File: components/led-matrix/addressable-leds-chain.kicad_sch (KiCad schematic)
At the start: 90 parts

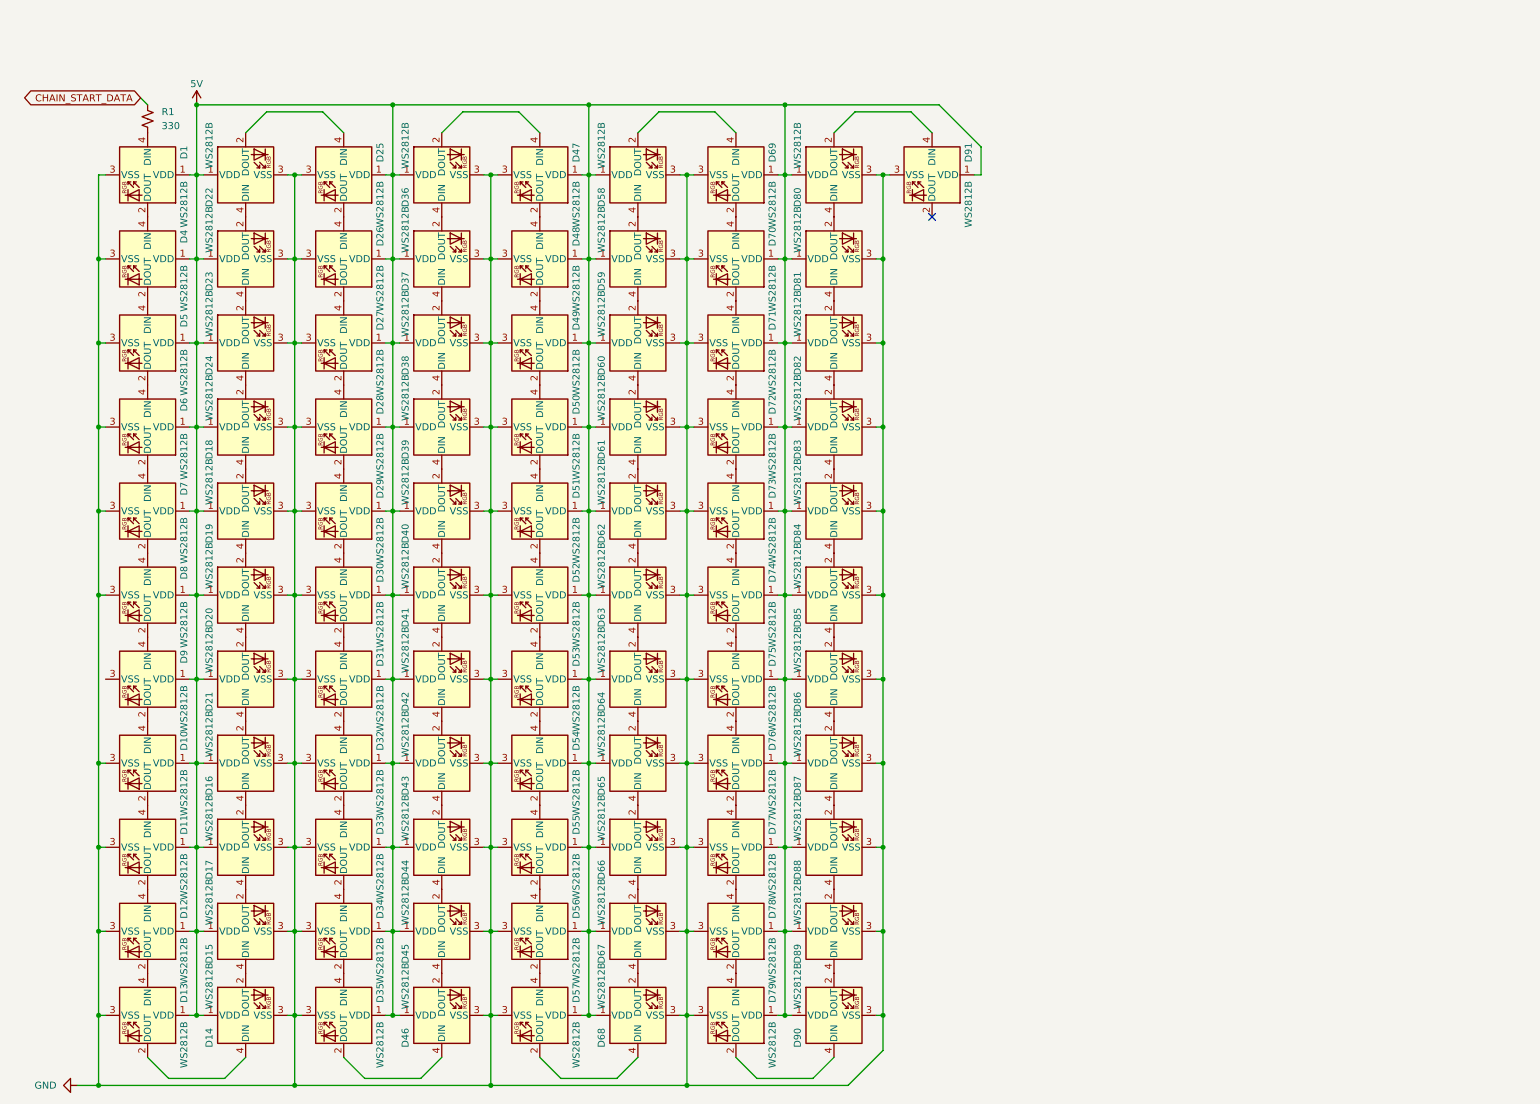
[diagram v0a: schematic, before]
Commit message: svg
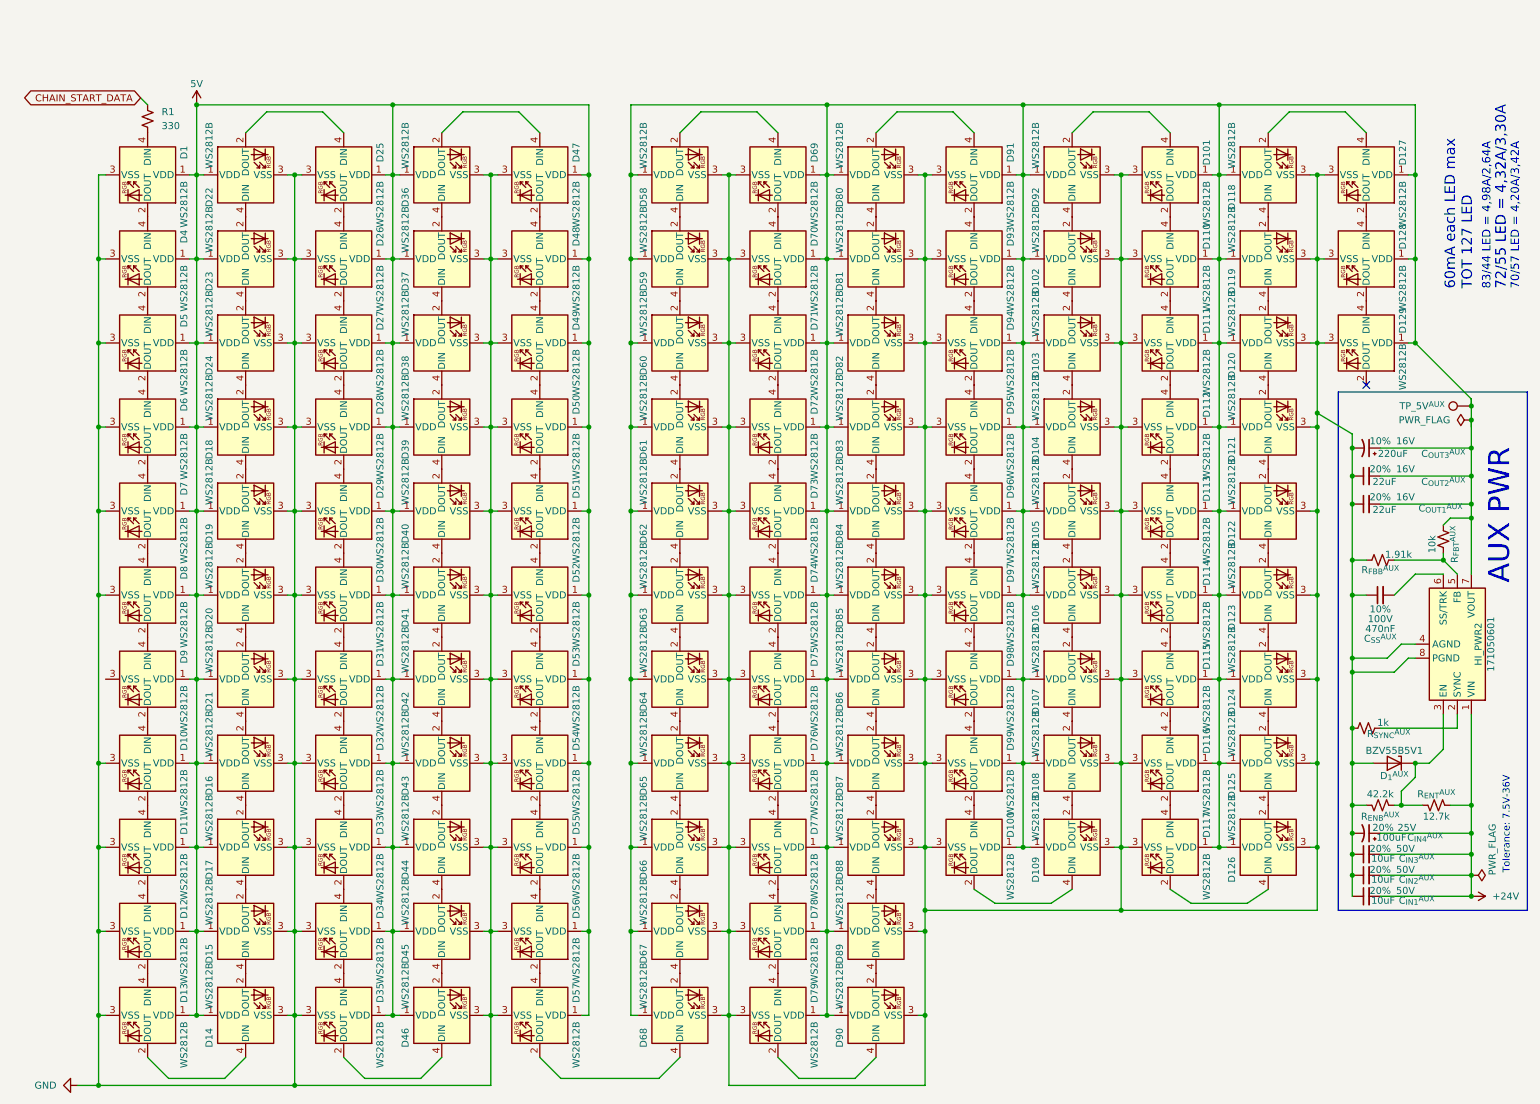
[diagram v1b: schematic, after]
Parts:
- added C_{IN1}^{AUX}, C_{IN2}^{AUX}, C_{IN3}^{AUX}: 10uF, PCM_SparkFun-Capacitor:C_1210_3225Metric, symbol PCM_SparkFun-Capacitor:10uF_1210_50V_20%
- added C_{IN4}^{AUX}: 100uF, PCM_SparkFun-Capacitor:Panasonic_D, symbol PCM_SparkFun-Capacitor:100uF_6.6x6.6_25V_20%
- added C_{OUT1}^{AUX}, C_{OUT2}^{AUX}: 22uF, PCM_SparkFun-Capacitor:C_0603_1608Metric, symbol PCM_SparkFun-Capacitor:22uF_0603_6.3V_20%
- added C_{OUT3}^{AUX}: 220uF, PCM_SparkFun-Capacitor:EIA-3528, symbol PCM_SparkFun-Capacitor:47uF_3528_10V_10%
- added C_{SS}^{AUX}: 470nF, PCM_SparkFun-Capacitor:C_0805_2012Metric, symbol PCM_SparkFun-Capacitor:470nF_0805_100V_10%
- added D100, D101, D102, D103, D104, D105, D106, D107, D108, D109, D110, D111, D112, D113, D114, D115, D116, D117, D118, D119, D120, D121, D122, D123, D124, D125, D126, D127, D128, D129, D92, D93, D94, D95, D96, D97, D98, D99: WS2812B, LED_SMD:LED_WS2812B_PLCC4_5.0x5.0mm_P3.2mm, symbol LED:WS2812B
- added D_{1}^{AUX}: BZV55B5V1, Diode_SMD:D_MiniMELF, symbol Diode:BZV55B5V1
- added HI_PWR2: 171050601, Package_TO_SOT_SMD:TO-263-7_TabPin8, symbol Regulator_Switching:171050601
- added R_{ENB}^{AUX}: 42.2k, PCM_SparkFun-Resistor:R_0603_1608Metric, symbol PCM_SparkFun-Resistor:12.4k_0603
- added R_{ENT}^{AUX}: 12.7k, PCM_SparkFun-Resistor:R_0603_1608Metric, symbol PCM_SparkFun-Resistor:12.4k_0603
- added R_{FBB}^{AUX}: 1.91k, PCM_SparkFun-Resistor:R_0603_1608Metric, symbol PCM_SparkFun-Resistor:1k_0603
- added R_{FBT}^{AUX}: 10k, PCM_SparkFun-Resistor:R_0603_1608Metric, symbol PCM_SparkFun-Resistor:10k_0603
- added R_{SYNC}^{AUX}: 1k, PCM_SparkFun-Resistor:R_0603_1608Metric, symbol PCM_SparkFun-Resistor:1k_0603
- added TP_5V^{AUX}: (no value), PCM_SparkFun-Connector:TestPoint-1.0mm, symbol Connector:TestPoint
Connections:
- net 5V: no longer D58.1 (VDD), D59.1 (VDD), D60.1 (VDD), D61.1 (VDD), D62.1 (VDD), D63.1 (VDD), D64.1 (VDD), D65.1 (VDD), D66.1 (VDD), D67.1 (VDD), D68.1 (VDD), D69.1 (VDD), D70.1 (VDD), D71.1 (VDD), D72.1 (VDD), D73.1 (VDD), D74.1 (VDD), D75.1 (VDD), D76.1 (VDD), D77.1 (VDD), D78.1 (VDD), D79.1 (VDD), D80.1 (VDD), D81.1 (VDD), D82.1 (VDD), D83.1 (VDD), D84.1 (VDD), D85.1 (VDD), D86.1 (VDD), D87.1 (VDD), D88.1 (VDD), D89.1 (VDD), D90.1 (VDD), D91.1 (VDD)
- net GND: no longer D58.3 (VSS), D59.3 (VSS), D60.3 (VSS), D61.3 (VSS), D62.3 (VSS), D63.3 (VSS), D64.3 (VSS), D65.3 (VSS), D66.3 (VSS), D67.3 (VSS), D68.3 (VSS), D69.3 (VSS), D70.3 (VSS), D71.3 (VSS), D72.3 (VSS), D73.3 (VSS), D74.3 (VSS), D75.3 (VSS), D76.3 (VSS), D77.3 (VSS), D78.3 (VSS), D79.3 (VSS), D80.3 (VSS), D81.3 (VSS), D82.3 (VSS), D83.3 (VSS), D84.3 (VSS), D85.3 (VSS), D86.3 (VSS), D87.3 (VSS), D88.3 (VSS), D89.3 (VSS), D90.3 (VSS), D91.3 (VSS)
- net at D91.2 (DOUT): now also D93.4 (DIN)
- new net: C_{OUT1}^{AUX}.2, C_{OUT2}^{AUX}.2, C_{OUT3}^{AUX}.1, D100.1 (VDD), D101.1 (VDD), D102.1 (VDD), D103.1 (VDD), D104.1 (VDD), D105.1 (VDD), D106.1 (VDD), D107.1 (VDD), D108.1 (VDD), D109.1 (VDD), D110.1 (VDD), D111.1 (VDD), D112.1 (VDD), D113.1 (VDD), D114.1 (VDD), D115.1 (VDD), D116.1 (VDD), D117.1 (VDD), D118.1 (VDD), D119.1 (VDD), D120.1 (VDD), D121.1 (VDD), D122.1 (VDD), D123.1 (VDD), D124.1 (VDD), D125.1 (VDD), D126.1 (VDD), D127.1 (VDD), D128.1 (VDD), D129.1 (VDD), D58.1 (VDD), D59.1 (VDD), D60.1 (VDD), D61.1 (VDD), D62.1 (VDD), D63.1 (VDD), D64.1 (VDD), D65.1 (VDD), D66.1 (VDD), D67.1 (VDD), D68.1 (VDD), D69.1 (VDD), D70.1 (VDD), D71.1 (VDD), D72.1 (VDD), D73.1 (VDD), D74.1 (VDD), D75.1 (VDD), D76.1 (VDD), D77.1 (VDD), D78.1 (VDD), D79.1 (VDD), D80.1 (VDD), D81.1 (VDD), D82.1 (VDD), D83.1 (VDD), D84.1 (VDD), D85.1 (VDD), D86.1 (VDD), D87.1 (VDD), D88.1 (VDD), D89.1 (VDD), D90.1 (VDD), D91.1 (VDD), D92.1 (VDD), D93.1 (VDD), D94.1 (VDD), D95.1 (VDD), D96.1 (VDD), D97.1 (VDD), D98.1 (VDD), D99.1 (VDD), HI_PWR2.7 (VOUT), R_{FBT}^{AUX}.1, TP_5V^{AUX}.1
- new net: C_{IN1}^{AUX}.1, C_{IN2}^{AUX}.1, C_{IN3}^{AUX}.1, C_{IN4}^{AUX}.2, C_{OUT1}^{AUX}.1, C_{OUT2}^{AUX}.1, C_{OUT3}^{AUX}.2, C_{SS}^{AUX}.1, D100.3 (VSS), D101.3 (VSS), D102.3 (VSS), D103.3 (VSS), D104.3 (VSS), D105.3 (VSS), D106.3 (VSS), D107.3 (VSS), D108.3 (VSS), D109.3 (VSS), D110.3 (VSS), D111.3 (VSS), D112.3 (VSS), D113.3 (VSS), D114.3 (VSS), D115.3 (VSS), D116.3 (VSS), D117.3 (VSS), D118.3 (VSS), D119.3 (VSS), D120.3 (VSS), D121.3 (VSS), D122.3 (VSS), D123.3 (VSS), D124.3 (VSS), D125.3 (VSS), D126.3 (VSS), D127.3 (VSS), D128.3 (VSS), D129.3 (VSS), D58.3 (VSS), D59.3 (VSS), D60.3 (VSS), D61.3 (VSS), D62.3 (VSS), D63.3 (VSS), D64.3 (VSS), D65.3 (VSS), D66.3 (VSS), D67.3 (VSS), D68.3 (VSS), D69.3 (VSS), D70.3 (VSS), D71.3 (VSS), D72.3 (VSS), D73.3 (VSS), D74.3 (VSS), D75.3 (VSS), D76.3 (VSS), D77.3 (VSS), D78.3 (VSS), D79.3 (VSS), D80.3 (VSS), D81.3 (VSS), D82.3 (VSS), D83.3 (VSS), D84.3 (VSS), D85.3 (VSS), D86.3 (VSS), D87.3 (VSS), D88.3 (VSS), D89.3 (VSS), D90.3 (VSS), D91.3 (VSS), D92.3 (VSS), D93.3 (VSS), D94.3 (VSS), D95.3 (VSS), D96.3 (VSS), D97.3 (VSS), D98.3 (VSS), D99.3 (VSS), D_{1}^{AUX}.2 (A), HI_PWR2.4 (AGND), HI_PWR2.8 (PGND), R_{ENB}^{AUX}.1, R_{FBB}^{AUX}.2, R_{SYNC}^{AUX}.1
- new net: D112.2 (DOUT), D113.4 (DIN)
- new net: D111.2 (DOUT), D112.4 (DIN)
- new net: D93.2 (DOUT), D94.4 (DIN)
- new net: D120.4 (DIN), D121.2 (DOUT)
- new net: D121.4 (DIN), D122.2 (DOUT)
- new net: D107.4 (DIN), D108.2 (DOUT)
- new net: D108.4 (DIN), D109.2 (DOUT)
- new net: D101.4 (DIN), D92.2 (DOUT)
- new net: D102.2 (DOUT), D92.4 (DIN)
- new net: HI_PWR2.5 (FB), R_{FBB}^{AUX}.1, R_{FBT}^{AUX}.2
- new net: D102.4 (DIN), D103.2 (DOUT)
- new net: D103.4 (DIN), D104.2 (DOUT)
- new net: HI_PWR2.2 (SYNC), R_{SYNC}^{AUX}.2
- new net: D_{1}^{AUX}.1 (K), HI_PWR2.3 (EN), R_{ENB}^{AUX}.2, R_{ENT}^{AUX}.2
- new net: C_{SS}^{AUX}.2, HI_PWR2.6 (SS/TRK)
- new net: D116.2 (DOUT), D117.4 (DIN)
- new net: D115.2 (DOUT), D116.4 (DIN)
- new net: D98.2 (DOUT), D99.4 (DIN)
- new net: D97.2 (DOUT), D98.4 (DIN)
- new net: D96.2 (DOUT), D97.4 (DIN)
- new net: D100.2 (DOUT), D109.4 (DIN)
- new net: D114.2 (DOUT), D115.4 (DIN)
- new net: D122.4 (DIN), D123.2 (DOUT)
- new net: D118.4 (DIN), D119.2 (DOUT)
- new net: D119.4 (DIN), D120.2 (DOUT)
- new net: D101.2 (DOUT), D110.4 (DIN)
- new net: D110.2 (DOUT), D111.4 (DIN)
- new net: D128.2 (DOUT), D129.4 (DIN)
- new net: D127.2 (DOUT), D128.4 (DIN)
- new net: D94.2 (DOUT), D95.4 (DIN)
- new net: D113.2 (DOUT), D114.4 (DIN)
- new net: D95.2 (DOUT), D96.4 (DIN)
- new net: D123.4 (DIN), D124.2 (DOUT)
- new net: D124.4 (DIN), D125.2 (DOUT)
- new net: D125.4 (DIN), D126.2 (DOUT)
- new net: D118.2 (DOUT), D127.4 (DIN)
- new net: D100.4 (DIN), D99.2 (DOUT)
- new net: D117.2 (DOUT), D126.4 (DIN)
- new net: D104.4 (DIN), D105.2 (DOUT)
- new net: D105.4 (DIN), D106.2 (DOUT)
- new net: D106.4 (DIN), D107.2 (DOUT)
- new net +24V: C_{IN1}^{AUX}.2, C_{IN2}^{AUX}.2, C_{IN3}^{AUX}.2, C_{IN4}^{AUX}.1, HI_PWR2.1 (VIN), R_{ENT}^{AUX}.1
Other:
- note added: "60mA each LED max TOT 127 LED _{83/44 LED = 4,98A/2,64A} 72/55 LED = 4,32A/3,30A ^{70/57 LED = 4,20A/3,42A}"
- note added: "AUX PWR"
- note added: "Tolerance: 7.5V-36V"
